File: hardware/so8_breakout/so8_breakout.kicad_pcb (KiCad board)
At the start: 2 copper layers, 15.7 x 10.7 mm, 3 parts, among them P1 CONN_4, P2 so8, P3 CONN_4

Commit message: moved modules
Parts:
- moved P1 412.6 mm to (376.2, 248.2)
- moved P2 412.6 mm to (380.6, 248.2)
- moved P3 412.6 mm to (388.9, 248.2)
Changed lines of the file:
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@@
     (links 8)
     (no_connects 0)
-    (area 0 0 0 0)
+    (area 27.619 17.450999 46.295 28.338214)
     (thickness 1.6)
     (drawings 5)
@@
     (pad_to_mask_clearance 0)
     (aux_axis_origin 0 0)
-    (visible_elements FFFFFFBF)
+    (visible_elements 7FFFFFFF)
     (pcbplotparams
       (layerselection 3178497)
@@
   )
   (module Stiftleiste_4x1 (layer F.Cu)
-    (at 43.18 22.86 90)
+    (at 388.874 248.158 90)
     (fp_text reference P3 (at 0 -2.032 90) (layer F.SilkS)
       (effects (font (size 1 1) (thickness 0.15)))
@@
   )
   (module Stiftleiste_4x1 (layer F.Cu)
-    (at 30.48 22.86 90)
+    (at 376.174 248.158 90)
     (fp_text reference P1 (at 0 -2.032 90) (layer F.SilkS)
       (effects (font (size 1 1) (thickness 0.15)))
@@
   )
   (module st485 (layer F.Cu)
-    (at 34.9377 22.86 90)
+    (at 380.6317 248.158 90)
     (descr st485)
     (attr smd)
@@
     )
   )
-  (gr_text SO8 (at 36.83 26.924) (layer F.Cu)
+  (gr_text SO8 (at 382.524 252.222) (layer F.Cu)
     (effects (font (size 1.5 1.5) (thickness 0.3)))
   )
-  (gr_line (start 28.956 28.194) (end 28.956 17.526) (angle 90) (layer Edge.Cuts) (width 0.1))
-  (gr_line (start 44.704 28.194) (end 28.956 28.194) (angle 90) (layer Edge.Cuts) (width 0.1))
-  (gr_line (start 44.704 17.526) (end 44.704 28.194) (angle 90) (layer Edge.Cuts) (width 0.1))
-  (gr_line (start 28.956 17.526) (end 44.704 17.526) (angle 90) (layer Edge.Cuts) (width 0.1))
-  (segment (start 33.7377 22.228) (end 32.4642 22.228) (width 0.6) (layer F.Cu) (net 1) (status 400000))
-  (segment (start 31.8262 21.59) (end 30.48 21.59) (width 0.6) (layer F.Cu) (net 1) (status 800000))
-  (segment (start 32.4642 22.228) (end 31.8262 21.59) (width 0.6) (layer F.Cu) (net 1))
-  (segment (start 40.0377 20.958) (end 40.9037 20.958) (width 0.6) (layer F.Cu) (net 2) (status C00000))
-  (segment (start 41.9862 19.05) (end 43.18 19.05) (width 0.6) (layer F.Cu) (net 2) (status 800000))
-  (segment (start 41.6306 19.4056) (end 41.9862 19.05) (width 0.6) (layer F.Cu) (net 2))
-  (segment (start 41.6306 20.2311) (end 41.6306 19.4056) (width 0.6) (layer F.Cu) (net 2))
-  (segment (start 40.9037 20.958) (end 41.6306 20.2311) (width 0.6) (layer F.Cu) (net 2) (status 400000))
-  (segment (start 40.0377 22.228) (end 41.4879 22.228) (width 0.6) (layer F.Cu) (net 3) (status 400000))
-  (segment (start 42.1259 21.59) (end 43.18 21.59) (width 0.6) (layer F.Cu) (net 3) (status 800000))
-  (segment (start 41.4879 22.228) (end 42.1259 21.59) (width 0.6) (layer F.Cu) (net 3))
-  (segment (start 33.7377 20.958) (end 32.6801 20.958) (width 0.6) (layer F.Cu) (net 4) (status 400000))
-  (segment (start 31.6738 19.05) (end 30.48 19.05) (width 0.6) (layer F.Cu) (net 4) (status 800000))
-  (segment (start 32.2961 19.6723) (end 31.6738 19.05) (width 0.6) (layer F.Cu) (net 4))
-  (segment (start 32.2961 20.574) (end 32.2961 19.6723) (width 0.6) (layer F.Cu) (net 4))
-  (segment (start 32.6801 20.958) (end 32.2961 20.574) (width 0.6) (layer F.Cu) (net 4))
-  (segment (start 33.7377 23.498) (end 32.2677 23.498) (width 0.6) (layer F.Cu) (net 5) (status 400000))
-  (segment (start 31.6357 24.13) (end 30.48 24.13) (width 0.6) (layer F.Cu) (net 5) (status 800000))
-  (segment (start 32.2677 23.498) (end 31.6357 24.13) (width 0.6) (layer F.Cu) (net 5))
-  (segment (start 33.7377 24.768) (end 32.89 24.768) (width 0.6) (layer F.Cu) (net 6) (status C00000))
-  (segment (start 31.4452 26.67) (end 30.48 26.67) (width 0.6) (layer F.Cu) (net 6) (status C00000))
-  (segment (start 32.0802 26.035) (end 31.4452 26.67) (width 0.6) (layer F.Cu) (net 6) (status 800000))
-  (segment (start 32.0802 25.5778) (end 32.0802 26.035) (width 0.6) (layer F.Cu) (net 6))
-  (segment (start 32.89 24.768) (end 32.0802 25.5778) (width 0.6) (layer F.Cu) (net 6) (status 400000))
-  (segment (start 40.0377 23.498) (end 41.6463 23.498) (width 0.6) (layer F.Cu) (net 7) (status 400000))
-  (segment (start 42.2783 24.13) (end 43.18 24.13) (width 0.6) (layer F.Cu) (net 7) (status C00000))
-  (segment (start 41.6463 23.498) (end 42.2783 24.13) (width 0.6) (layer F.Cu) (net 7) (status 800000))
-  (segment (start 40.0377 24.768) (end 41.1891 24.768) (width 0.6) (layer F.Cu) (net 8) (status 400000))
-  (segment (start 41.9354 26.67) (end 43.18 26.67) (width 0.6) (layer F.Cu) (net 8) (status 800000))
-  (segment (start 41.5163 26.2509) (end 41.9354 26.67) (width 0.6) (layer F.Cu) (net 8))
-  (segment (start 41.5163 25.0952) (end 41.5163 26.2509) (width 0.6) (layer F.Cu) (net 8))
-  (segment (start 41.1891 24.768) (end 41.5163 25.0952) (width 0.6) (layer F.Cu) (net 8))
+  (gr_line (start 374.65 253.492) (end 374.65 242.824) (angle 90) (layer Edge.Cuts) (width 0.1))
+  (gr_line (start 390.398 253.492) (end 374.65 253.492) (angle 90) (layer Edge.Cuts) (width 0.1))
+  (gr_line (start 390.398 242.824) (end 390.398 253.492) (angle 90) (layer Edge.Cuts) (width 0.1))
+  (gr_line (start 374.65 242.824) (end 390.398 242.824) (angle 90) (layer Edge.Cuts) (width 0.1))
+  (segment (start 379.4317 247.526) (end 378.1582 247.526) (width 0.6) (layer F.Cu) (net 1))
+  (segment (start 377.5202 246.888) (end 376.174 246.888) (width 0.6) (layer F.Cu) (net 1))
+  (segment (start 378.1582 247.526) (end 377.5202 246.888) (width 0.6) (layer F.Cu) (net 1))
+  (segment (start 385.7317 246.256) (end 386.5977 246.256) (width 0.6) (layer F.Cu) (net 2))
+  (segment (start 387.6802 244.348) (end 388.874 244.348) (width 0.6) (layer F.Cu) (net 2))
+  (segment (start 387.3246 244.7036) (end 387.6802 244.348) (width 0.6) (layer F.Cu) (net 2))
+  (segment (start 387.3246 245.5291) (end 387.3246 244.7036) (width 0.6) (layer F.Cu) (net 2))
+  (segment (start 386.5977 246.256) (end 387.3246 245.5291) (width 0.6) (layer F.Cu) (net 2))
+  (segment (start 385.7317 247.526) (end 387.1819 247.526) (width 0.6) (layer F.Cu) (net 3))
+  (segment (start 387.8199 246.888) (end 388.874 246.888) (width 0.6) (layer F.Cu) (net 3))
+  (segment (start 387.1819 247.526) (end 387.8199 246.888) (width 0.6) (layer F.Cu) (net 3))
+  (segment (start 379.4317 246.256) (end 378.3741 246.256) (width 0.6) (layer F.Cu) (net 4))
+  (segment (start 377.3678 244.348) (end 376.174 244.348) (width 0.6) (layer F.Cu) (net 4))
+  (segment (start 377.9901 244.9703) (end 377.3678 244.348) (width 0.6) (layer F.Cu) (net 4))
+  (segment (start 377.9901 245.872) (end 377.9901 244.9703) (width 0.6) (layer F.Cu) (net 4))
+  (segment (start 378.3741 246.256) (end 377.9901 245.872) (width 0.6) (layer F.Cu) (net 4))
+  (segment (start 379.4317 248.796) (end 377.9617 248.796) (width 0.6) (layer F.Cu) (net 5))
+  (segment (start 377.3297 249.428) (end 376.174 249.428) (width 0.6) (layer F.Cu) (net 5))
+  (segment (start 377.9617 248.796) (end 377.3297 249.428) (width 0.6) (layer F.Cu) (net 5))
+  (segment (start 379.4317 250.066) (end 378.584 250.066) (width 0.6) (layer F.Cu) (net 6))
+  (segment (start 377.1392 251.968) (end 376.174 251.968) (width 0.6) (layer F.Cu) (net 6))
+  (segment (start 377.7742 251.333) (end 377.1392 251.968) (width 0.6) (layer F.Cu) (net 6))
+  (segment (start 377.7742 250.8758) (end 377.7742 251.333) (width 0.6) (layer F.Cu) (net 6))
+  (segment (start 378.584 250.066) (end 377.7742 250.8758) (width 0.6) (layer F.Cu) (net 6))
+  (segment (start 385.7317 248.796) (end 387.3403 248.796) (width 0.6) (layer F.Cu) (net 7))
+  (segment (start 387.9723 249.428) (end 388.874 249.428) (width 0.6) (layer F.Cu) (net 7))
+  (segment (start 387.3403 248.796) (end 387.9723 249.428) (width 0.6) (layer F.Cu) (net 7))
+  (segment (start 385.7317 250.066) (end 386.8831 250.066) (width 0.6) (layer F.Cu) (net 8))
+  (segment (start 387.6294 251.968) (end 388.874 251.968) (width 0.6) (layer F.Cu) (net 8))
+  (segment (start 387.2103 251.5489) (end 387.6294 251.968) (width 0.6) (layer F.Cu) (net 8))
+  (segment (start 387.2103 250.3932) (end 387.2103 251.5489) (width 0.6) (layer F.Cu) (net 8))
+  (segment (start 386.8831 250.066) (end 387.2103 250.3932) (width 0.6) (layer F.Cu) (net 8))
 )

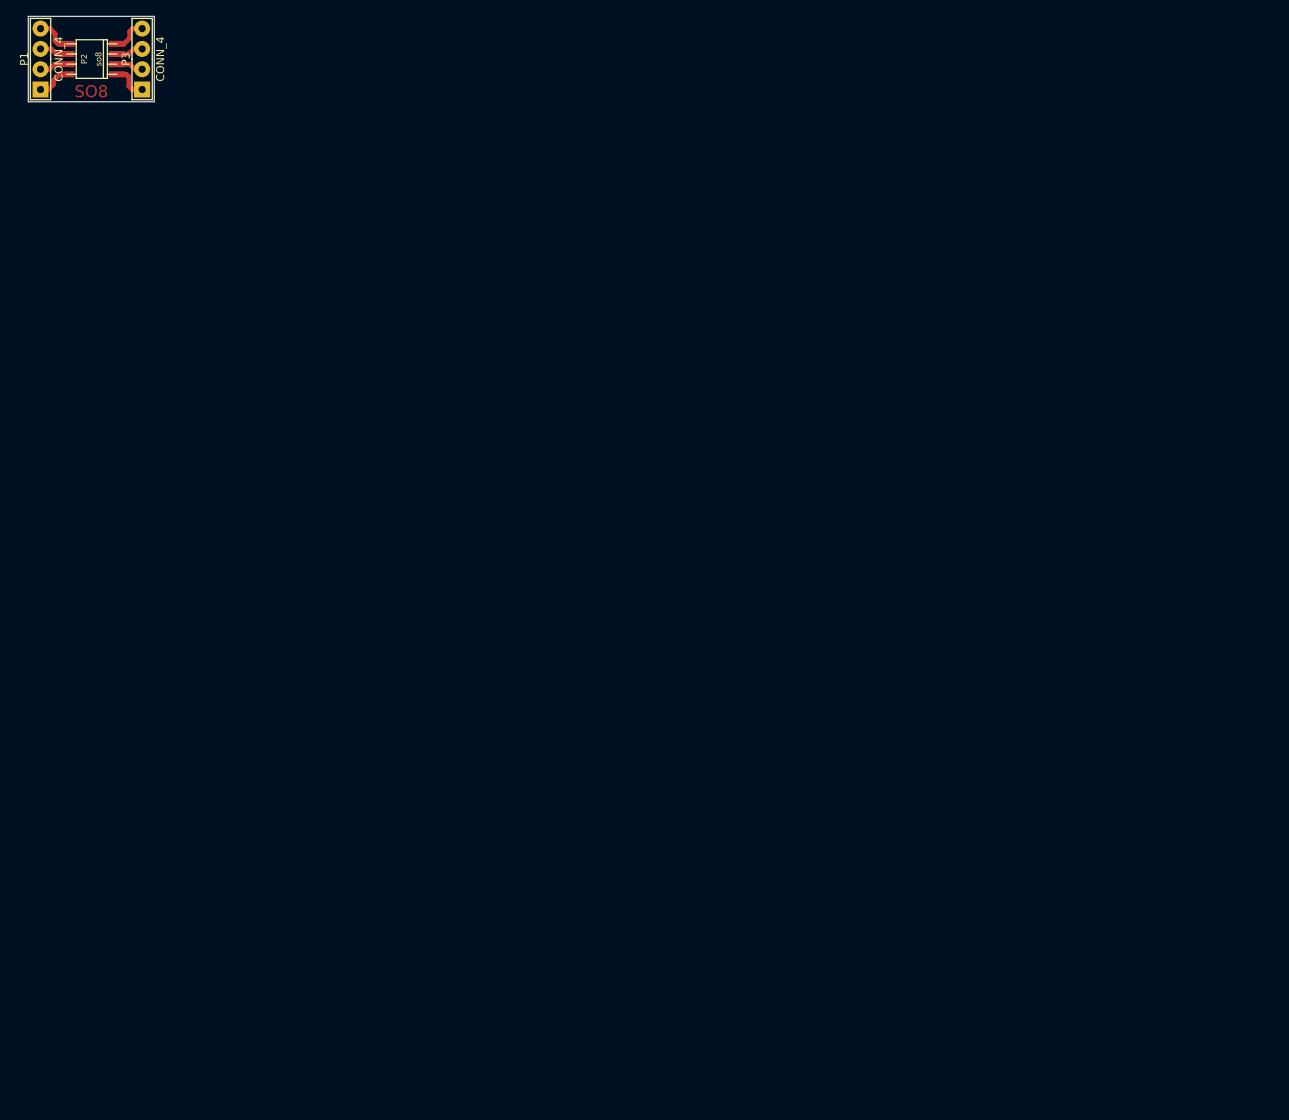
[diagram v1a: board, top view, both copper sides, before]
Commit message: a little modification
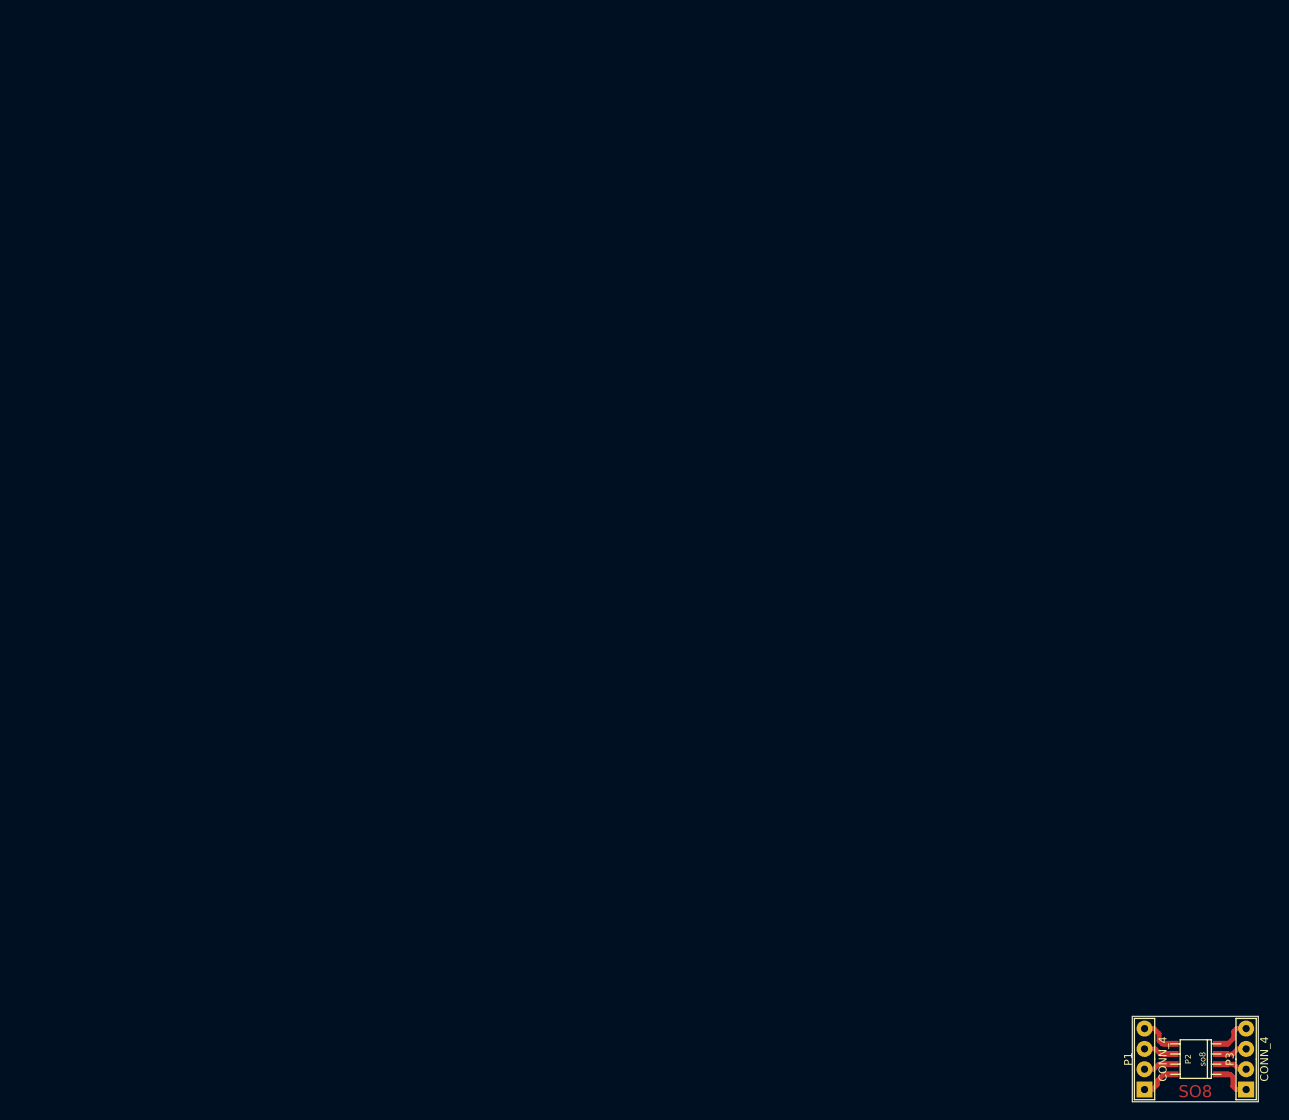
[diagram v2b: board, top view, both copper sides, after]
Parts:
- moved P1 186.2 mm to (514.2, 373.2)
- moved P2 186.2 mm to (518.6, 373.2)
- moved P3 186.2 mm to (526.9, 373.2)
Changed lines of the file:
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@@
     (links 8)
     (no_connects 0)
-    (area 27.619 17.450999 46.295 28.338214)
+    (area 373.313 242.748999 391.989 253.636214)
     (thickness 1.6)
     (drawings 5)
@@
     (nets 9)
   )
-  (page A3)
+  (page A2)
   (layers
     (15 F.Cu signal)
@@
   )
   (module Stiftleiste_4x1 (layer F.Cu)
-    (at 388.874 248.158 90)
+    (at 526.874 373.158 90)
     (fp_text reference P3 (at 0 -2.032 90) (layer F.SilkS)
       (effects (font (size 1 1) (thickness 0.15)))
@@
   )
   (module Stiftleiste_4x1 (layer F.Cu)
-    (at 376.174 248.158 90)
+    (at 514.174 373.158 90)
     (fp_text reference P1 (at 0 -2.032 90) (layer F.SilkS)
       (effects (font (size 1 1) (thickness 0.15)))
@@
   )
   (module st485 (layer F.Cu)
-    (at 380.6317 248.158 90)
+    (at 518.6317 373.158 90)
     (descr st485)
     (attr smd)
@@
     )
   )
-  (gr_text SO8 (at 382.524 252.222) (layer F.Cu)
+  (gr_text SO8 (at 520.524 377.222) (layer F.Cu)
     (effects (font (size 1.5 1.5) (thickness 0.3)))
   )
-  (gr_line (start 374.65 253.492) (end 374.65 242.824) (angle 90) (layer Edge.Cuts) (width 0.1))
-  (gr_line (start 390.398 253.492) (end 374.65 253.492) (angle 90) (layer Edge.Cuts) (width 0.1))
-  (gr_line (start 390.398 242.824) (end 390.398 253.492) (angle 90) (layer Edge.Cuts) (width 0.1))
-  (gr_line (start 374.65 242.824) (end 390.398 242.824) (angle 90) (layer Edge.Cuts) (width 0.1))
-  (segment (start 379.4317 247.526) (end 378.1582 247.526) (width 0.6) (layer F.Cu) (net 1))
-  (segment (start 377.5202 246.888) (end 376.174 246.888) (width 0.6) (layer F.Cu) (net 1))
-  (segment (start 378.1582 247.526) (end 377.5202 246.888) (width 0.6) (layer F.Cu) (net 1))
-  (segment (start 385.7317 246.256) (end 386.5977 246.256) (width 0.6) (layer F.Cu) (net 2))
-  (segment (start 387.6802 244.348) (end 388.874 244.348) (width 0.6) (layer F.Cu) (net 2))
-  (segment (start 387.3246 244.7036) (end 387.6802 244.348) (width 0.6) (layer F.Cu) (net 2))
-  (segment (start 387.3246 245.5291) (end 387.3246 244.7036) (width 0.6) (layer F.Cu) (net 2))
-  (segment (start 386.5977 246.256) (end 387.3246 245.5291) (width 0.6) (layer F.Cu) (net 2))
-  (segment (start 385.7317 247.526) (end 387.1819 247.526) (width 0.6) (layer F.Cu) (net 3))
-  (segment (start 387.8199 246.888) (end 388.874 246.888) (width 0.6) (layer F.Cu) (net 3))
-  (segment (start 387.1819 247.526) (end 387.8199 246.888) (width 0.6) (layer F.Cu) (net 3))
-  (segment (start 379.4317 246.256) (end 378.3741 246.256) (width 0.6) (layer F.Cu) (net 4))
-  (segment (start 377.3678 244.348) (end 376.174 244.348) (width 0.6) (layer F.Cu) (net 4))
-  (segment (start 377.9901 244.9703) (end 377.3678 244.348) (width 0.6) (layer F.Cu) (net 4))
-  (segment (start 377.9901 245.872) (end 377.9901 244.9703) (width 0.6) (layer F.Cu) (net 4))
-  (segment (start 378.3741 246.256) (end 377.9901 245.872) (width 0.6) (layer F.Cu) (net 4))
-  (segment (start 379.4317 248.796) (end 377.9617 248.796) (width 0.6) (layer F.Cu) (net 5))
-  (segment (start 377.3297 249.428) (end 376.174 249.428) (width 0.6) (layer F.Cu) (net 5))
-  (segment (start 377.9617 248.796) (end 377.3297 249.428) (width 0.6) (layer F.Cu) (net 5))
-  (segment (start 379.4317 250.066) (end 378.584 250.066) (width 0.6) (layer F.Cu) (net 6))
-  (segment (start 377.1392 251.968) (end 376.174 251.968) (width 0.6) (layer F.Cu) (net 6))
-  (segment (start 377.7742 251.333) (end 377.1392 251.968) (width 0.6) (layer F.Cu) (net 6))
-  (segment (start 377.7742 250.8758) (end 377.7742 251.333) (width 0.6) (layer F.Cu) (net 6))
-  (segment (start 378.584 250.066) (end 377.7742 250.8758) (width 0.6) (layer F.Cu) (net 6))
-  (segment (start 385.7317 248.796) (end 387.3403 248.796) (width 0.6) (layer F.Cu) (net 7))
-  (segment (start 387.9723 249.428) (end 388.874 249.428) (width 0.6) (layer F.Cu) (net 7))
-  (segment (start 387.3403 248.796) (end 387.9723 249.428) (width 0.6) (layer F.Cu) (net 7))
-  (segment (start 385.7317 250.066) (end 386.8831 250.066) (width 0.6) (layer F.Cu) (net 8))
-  (segment (start 387.6294 251.968) (end 388.874 251.968) (width 0.6) (layer F.Cu) (net 8))
-  (segment (start 387.2103 251.5489) (end 387.6294 251.968) (width 0.6) (layer F.Cu) (net 8))
-  (segment (start 387.2103 250.3932) (end 387.2103 251.5489) (width 0.6) (layer F.Cu) (net 8))
-  (segment (start 386.8831 250.066) (end 387.2103 250.3932) (width 0.6) (layer F.Cu) (net 8))
+  (gr_line (start 512.65 378.492) (end 512.65 367.824) (angle 90) (layer Edge.Cuts) (width 0.1))
+  (gr_line (start 528.398 378.492) (end 512.65 378.492) (angle 90) (layer Edge.Cuts) (width 0.1))
+  (gr_line (start 528.398 367.824) (end 528.398 378.492) (angle 90) (layer Edge.Cuts) (width 0.1))
+  (gr_line (start 512.65 367.824) (end 528.398 367.824) (angle 90) (layer Edge.Cuts) (width 0.1))
+  (segment (start 517.4317 372.526) (end 516.1582 372.526) (width 0.6) (layer F.Cu) (net 1))
+  (segment (start 515.5202 371.888) (end 514.174 371.888) (width 0.6) (layer F.Cu) (net 1))
+  (segment (start 516.1582 372.526) (end 515.5202 371.888) (width 0.6) (layer F.Cu) (net 1))
+  (segment (start 523.7317 371.256) (end 524.5977 371.256) (width 0.6) (layer F.Cu) (net 2))
+  (segment (start 525.6802 369.348) (end 526.874 369.348) (width 0.6) (layer F.Cu) (net 2))
+  (segment (start 525.3246 369.7036) (end 525.6802 369.348) (width 0.6) (layer F.Cu) (net 2))
+  (segment (start 525.3246 370.5291) (end 525.3246 369.7036) (width 0.6) (layer F.Cu) (net 2))
+  (segment (start 524.5977 371.256) (end 525.3246 370.5291) (width 0.6) (layer F.Cu) (net 2))
+  (segment (start 523.7317 372.526) (end 525.1819 372.526) (width 0.6) (layer F.Cu) (net 3))
+  (segment (start 525.8199 371.888) (end 526.874 371.888) (width 0.6) (layer F.Cu) (net 3))
+  (segment (start 525.1819 372.526) (end 525.8199 371.888) (width 0.6) (layer F.Cu) (net 3))
+  (segment (start 517.4317 371.256) (end 516.3741 371.256) (width 0.6) (layer F.Cu) (net 4))
+  (segment (start 515.3678 369.348) (end 514.174 369.348) (width 0.6) (layer F.Cu) (net 4))
+  (segment (start 515.9901 369.9703) (end 515.3678 369.348) (width 0.6) (layer F.Cu) (net 4))
+  (segment (start 515.9901 370.872) (end 515.9901 369.9703) (width 0.6) (layer F.Cu) (net 4))
+  (segment (start 516.3741 371.256) (end 515.9901 370.872) (width 0.6) (layer F.Cu) (net 4))
+  (segment (start 517.4317 373.796) (end 515.9617 373.796) (width 0.6) (layer F.Cu) (net 5))
+  (segment (start 515.3297 374.428) (end 514.174 374.428) (width 0.6) (layer F.Cu) (net 5))
+  (segment (start 515.9617 373.796) (end 515.3297 374.428) (width 0.6) (layer F.Cu) (net 5))
+  (segment (start 517.4317 375.066) (end 516.584 375.066) (width 0.6) (layer F.Cu) (net 6))
+  (segment (start 515.1392 376.968) (end 514.174 376.968) (width 0.6) (layer F.Cu) (net 6))
+  (segment (start 515.7742 376.333) (end 515.1392 376.968) (width 0.6) (layer F.Cu) (net 6))
+  (segment (start 515.7742 375.8758) (end 515.7742 376.333) (width 0.6) (layer F.Cu) (net 6))
+  (segment (start 516.584 375.066) (end 515.7742 375.8758) (width 0.6) (layer F.Cu) (net 6))
+  (segment (start 523.7317 373.796) (end 525.3403 373.796) (width 0.6) (layer F.Cu) (net 7))
+  (segment (start 525.9723 374.428) (end 526.874 374.428) (width 0.6) (layer F.Cu) (net 7))
+  (segment (start 525.3403 373.796) (end 525.9723 374.428) (width 0.6) (layer F.Cu) (net 7))
+  (segment (start 523.7317 375.066) (end 524.8831 375.066) (width 0.6) (layer F.Cu) (net 8))
+  (segment (start 525.6294 376.968) (end 526.874 376.968) (width 0.6) (layer F.Cu) (net 8))
+  (segment (start 525.2103 376.5489) (end 525.6294 376.968) (width 0.6) (layer F.Cu) (net 8))
+  (segment (start 525.2103 375.3932) (end 525.2103 376.5489) (width 0.6) (layer F.Cu) (net 8))
+  (segment (start 524.8831 375.066) (end 525.2103 375.3932) (width 0.6) (layer F.Cu) (net 8))
 )
